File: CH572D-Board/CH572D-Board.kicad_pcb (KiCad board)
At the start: 2 copper layers, 16.4 x 26.4 mm, 17 parts, among them J1 12402012E212A, J2 Conn_PinHeader_1x07_P2.54mm_V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, U2 the really cheap one (200mah), Y1 32mhz

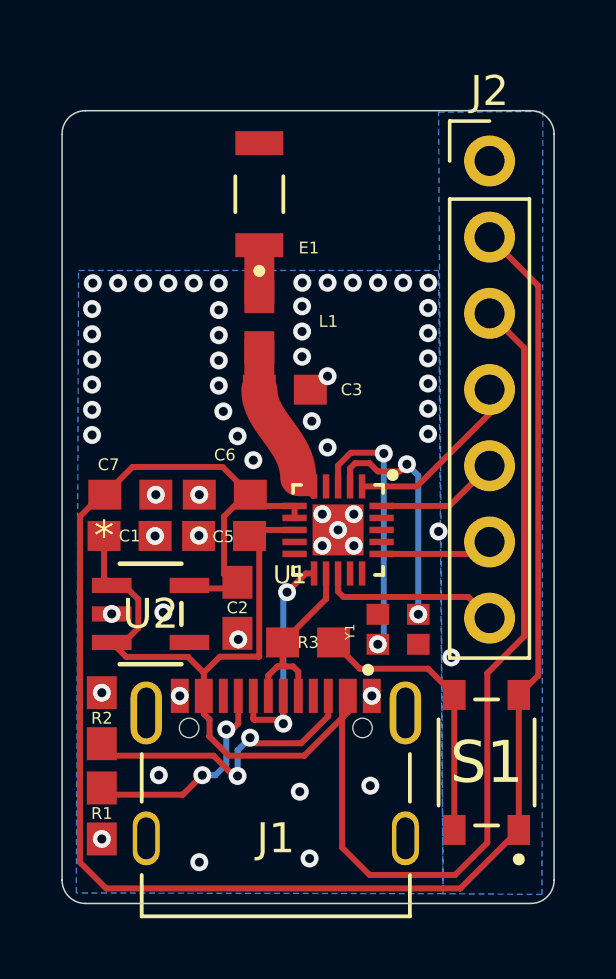
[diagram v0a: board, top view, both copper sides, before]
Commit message: redid and reordered
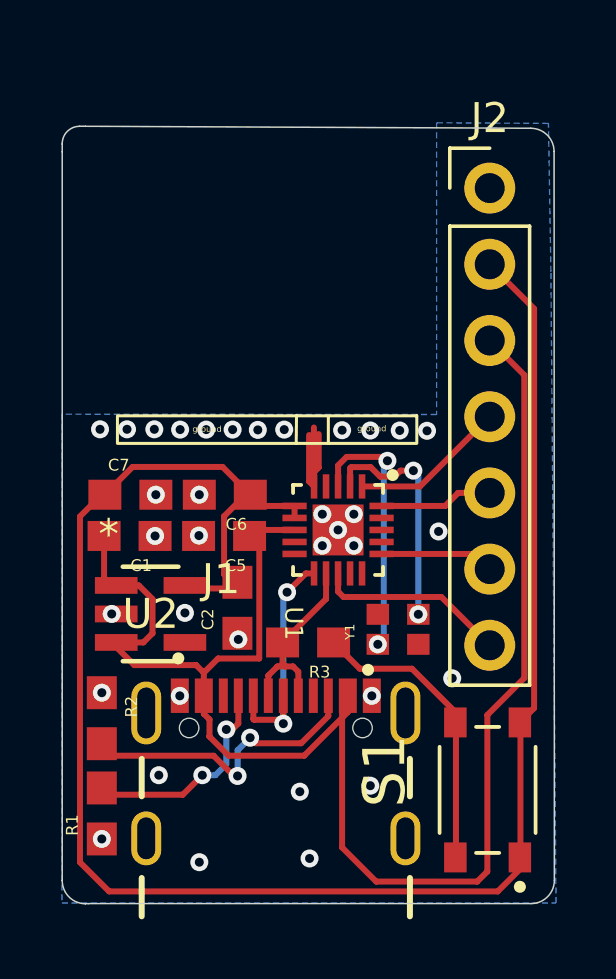
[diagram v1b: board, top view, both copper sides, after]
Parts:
- removed C3: 1.5pF, Personal:0603
- removed L1: 3.9nH, Personal:0603
- C1, C2, C5, C6, C7, R1, R2, R3: footprint Personal:0603 -> Footprint:0603
- E1: footprint Personal:ceramic antenna -> Footprint:DM00024648
- J1: footprint usbcport:usbcport -> Footprint:usbc
- J2: footprint fab:PinHeader_1x07_P2.54mm_Vertical_THT_D1mm -> Footprint:PinHeader_01x07_P2.54mm_Vertical_THT_D1mm
- S1: footprint Personal:button -> Footprint:button
- U1: footprint Ch572D:CH572D -> Footprint:CH572D
- U2: footprint 300mah 3.3v vreg:SOT-23-5_MC_MCH -> Footprint:voltage regulator
- Y1: footprint Personal:32mhz crystal -> Footprint:32mhz crystal
- moved E1 4.72 mm to (159.9, 127.1), turned to 0 degrees
- moved S1 0.92 mm to (167.3, 142.2)
- moved J2 0.91 mm to (167.4, 122.2)
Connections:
- E1 pad 1: Net-(E1-Pad1) -> Net-(U1-ANT)
- U1 pad 5: ANTENNA -> Net-(U1-ANT)
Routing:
- net Net-(U1-ANT): track 0.00 -> 5.56 mm
- net +5V: track 53.8 -> 54.8 mm
- net PA3: track 6.06 -> 5.22 mm
- net ANTENNA: track 0.82 -> 0.00 mm
- net Net-(R3-Pad1): track 9.25 -> 9.86 mm
- net +3.3V: track 62.6 -> 62.1 mm
- net GND: track 0.07 -> 0.45 mm, vias 60 -> 35
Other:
- board size 16.4 x 26.4 mm -> 16.4 x 25.9 mm
